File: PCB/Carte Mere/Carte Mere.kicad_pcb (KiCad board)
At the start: 4 copper layers, 63.5 x 62.2 mm, 55 parts, among them J1 Alim 6V, J10 Conn_01x03_Male, J11 Conn_01x03_Male, J12 Conn_Tcrt5000, J13 Conn_Tcrt5000, J14 01x20_Female, J15 01x20_Female, J16 Conn_Tcrt5000, J17 Conn_Tcrt5000, J2 Alim 9V, J3 Moteur, J4 Moteur, J5 01x20_Female, J6 01x20_Female, J7 Conn_01x03_Male, J8 Conn_01x03_Male, J9 TL1838, U1 ZXBM5210-S, U2 MC33269DR2-5.0G, U3 ZXBM5210-S, U4 LD1117S33TR_SOT223, U5 TCRT5000, U6 TCRT5000, U7 TCRT5000, U8 TCRT5000

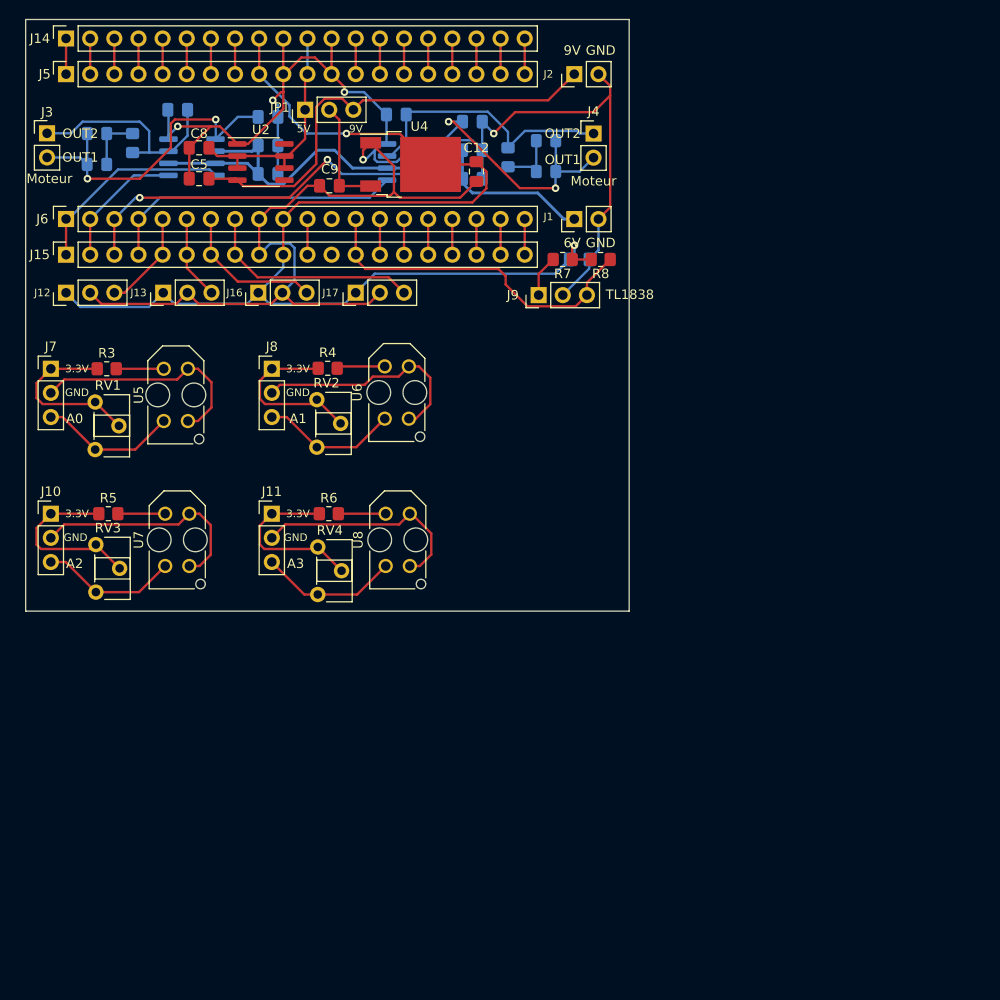
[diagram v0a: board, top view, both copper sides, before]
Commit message: Fixed Zach's errors :/ smh
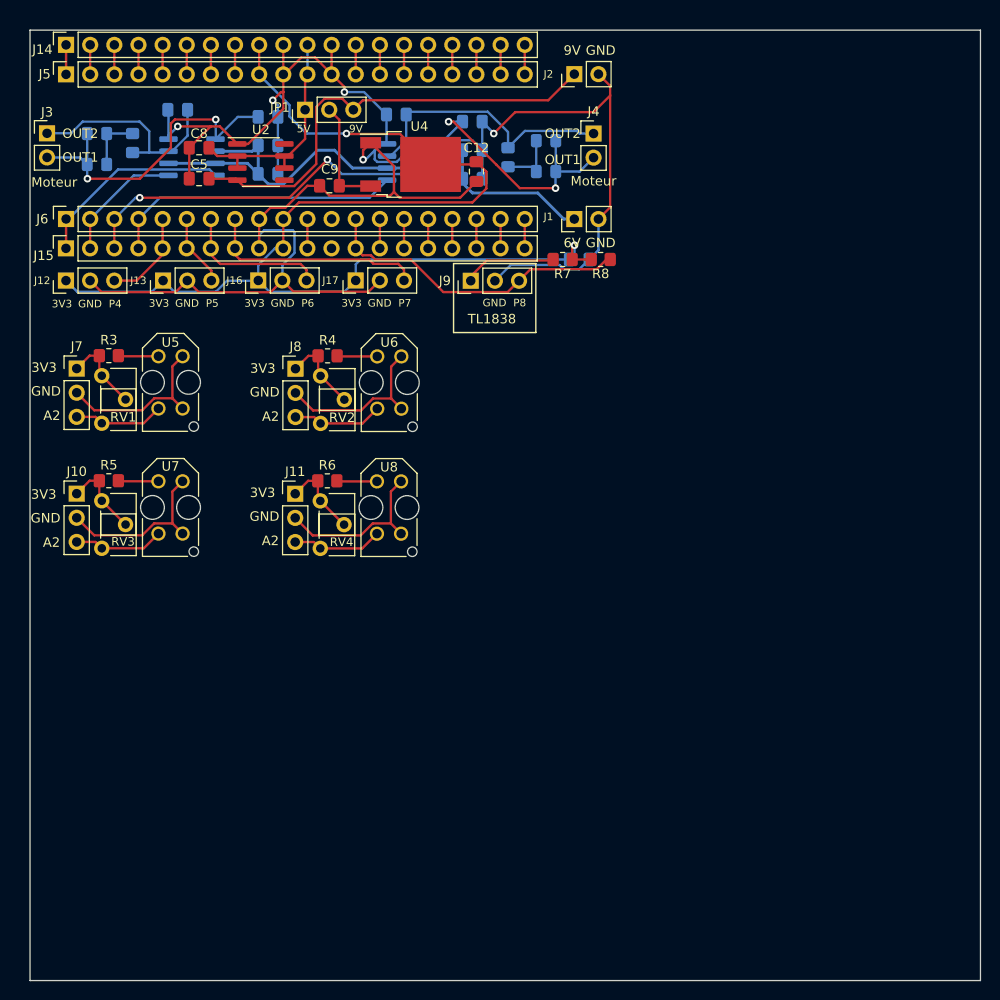
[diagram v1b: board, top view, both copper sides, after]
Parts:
- moved J9 7.30 mm to (145.8, 74.2)
- moved RV4 4.86 mm to (130.0, 97.4)
- moved RV3 4.65 mm to (107.0, 97.4)
- moved U8 3.52 mm to (137.2, 98.1)
- moved U7 3.48 mm to (114.2, 98.1)
- moved R5 3.47 mm to (107.8, 95.3)
- moved R6 3.46 mm to (130.7, 95.3)
- moved J10 3.44 mm to (104.4, 96.6)
- moved J11 3.23 mm to (127.4, 96.7)
- moved RV1 2.86 mm to (107.0, 84.2)
- moved J7 2.72 mm to (104.4, 83.5)
- moved RV2 2.53 mm to (130.0, 84.2)
- moved J8 2.49 mm to (127.4, 83.5)
- moved U5 1.43 mm to (114.2, 84.9)
- moved R3 1.40 mm to (107.8, 82.1)
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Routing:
- net 3.3V: track 203.8 -> 163.2 mm
- net GND: track 303.9 -> 285.8 mm
- net Net-(J9-Pad1): track 4.38 -> 9.87 mm
- net /Capteur/A3: track 14.6 -> 9.52 mm
- net /Capteur/A0: track 14.5 -> 9.52 mm
- net /Capteur/A2: track 14.5 -> 9.52 mm
- net /Capteur/A1: track 14.4 -> 9.52 mm
- net P8: track 36.4 -> 33.2 mm
- net /Carte Mere/P5: track 8.84 -> 7.71 mm
- net Net-(R4-Pad2): track 5.08 -> 4.24 mm
- net Net-(R3-Pad2): track 5.00 -> 4.24 mm
- net Net-(R5-Pad2): track 4.98 -> 4.24 mm
- net Net-(R6-Pad2): track 4.98 -> 4.24 mm
- net /Carte Mere/P15: track 3.76 -> 3.09 mm
- net /Carte Mere/P14: track 3.76 -> 3.09 mm
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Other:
- board size 63.5 x 62.2 mm -> 100 x 100 mm
- board text added: "3V3"
- board text added: "Conn_Tcrt5000"
- board text added: "P4"
- board text added: "P5"
- board text added: "P6"
- board text added: "P7"
- board text added: "P8"
- board text removed: "3.3V"
- board text removed: "A0"
- board text removed: "A1"
- board text removed: "A3"
